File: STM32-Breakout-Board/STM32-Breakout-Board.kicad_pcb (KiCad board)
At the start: 2 copper layers, 32 parts, among them J1 USB_B_Micro, J2 Conn_01x04_Pin, J3 Conn_01x10_Socket, J4 Conn_01x10_Socket, SW1 SW_SPDT, U1 stm32l443cct6, U2 MCP1799T-3302H/DB, Y1 Crystal_GND24

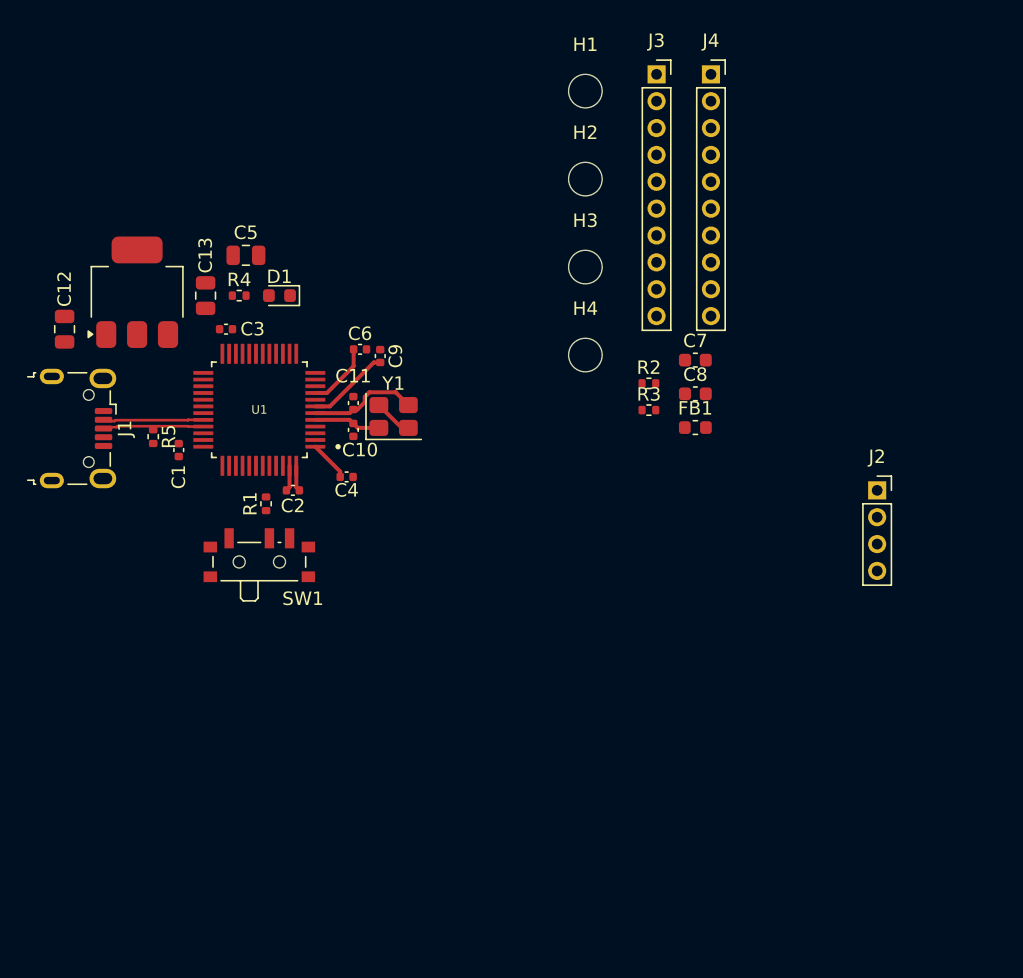
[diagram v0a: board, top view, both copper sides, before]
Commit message: Final Update
Completed layout and Silkscreen decoration
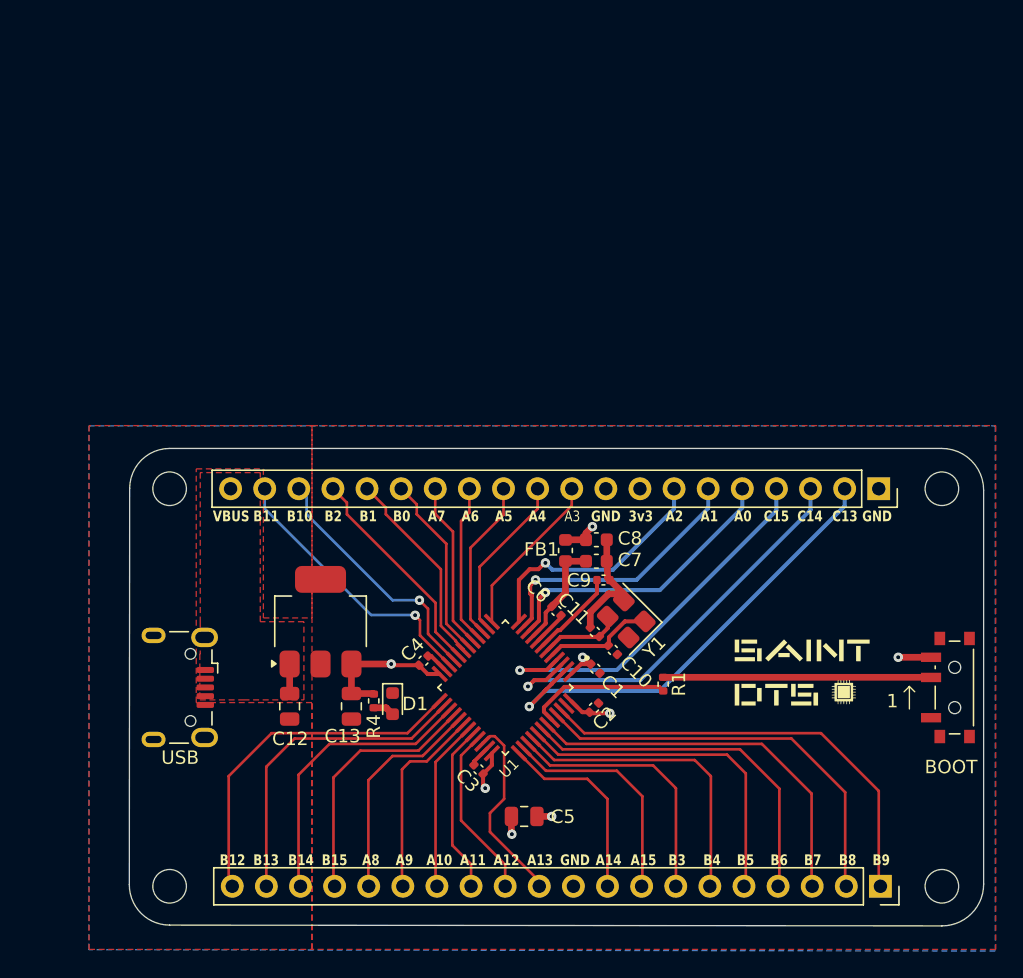
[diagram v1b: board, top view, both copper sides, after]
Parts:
- removed J1: USB_B_Micro, Connector_USB:USB_Micro-B_Wuerth_629105150521
- removed J4: Conn_01x10_Socket, Connector_PinSocket_2.00mm:PinSocket_1x10_P2.00mm_Vertical
- removed R2, R3, R5: 1k5, Resistor_SMD:R_0402_1005Metric
- removed SW1: SW_SPDT, Button_Switch_SMD:SW_SPDT_PCM12
- added BOOT: SW_SPDT, Button_Switch_SMD:SW_SPDT_PCM12, F.Cu at (180.9, 90.7)
- added G***: LOGO, LOGO, F.Cu at (169.9, 89.5)
- added USB: USB_B_Micro, Connector_USB:USB_Micro-B_Wuerth_629105150521, F.Cu at (123.6, 90.7)
- J2: value Conn_01x04_Pin -> Conn_01x20_Pin; footprint Connector_PinSocket_2.00mm:PinSocket_1x04_P2.00mm_Vertical -> Connector_PinHeader_2.54mm:PinHeader_1x20_P2.54mm_Vertical; moved to B.Cu
- J3: value Conn_01x10_Socket -> Conn_01x20_Pin; footprint Connector_PinSocket_2.00mm:PinSocket_1x10_P2.00mm_Vertical -> Connector_PinHeader_2.54mm:PinHeader_1x20_P2.54mm_Vertical; moved to B.Cu
- moved J3 62.7 mm to (175.7, 105.5), turned to 90 degrees
- moved H2 59.0 mm to (180.3, 105.5), turned to -90 degrees
- moved H3 55.5 mm to (122.8, 105.5), turned to -90 degrees
- moved C5 46.6 mm to (149.2, 100.3), turned to 180 degrees
- moved H1 39.8 mm to (180.3, 75.9), turned to -90 degrees
- moved C3 37.8 mm to (145.8, 96.8), turned to 135 degrees
- moved C1 35.0 mm to (154.5, 89.3), turned to -45 degrees
- moved C12 32.7 mm to (131.8, 92.1), turned to -90 degrees
- moved H4 32.5 mm to (122.8, 75.9), turned to -90 degrees
- moved R1 32.5 mm to (159.6, 90.4), turned to -90 degrees
- moved C13 32.4 mm to (136.4, 92.1), turned to -90 degrees
- moved R4 31.8 mm to (138.0, 91.7), turned to -90 degrees
- moved D1 31.5 mm to (139.4, 91.9), turned to -90 degrees
- moved U2 28.1 mm to (134.7, 85.9)
- moved C2 27.6 mm to (154.4, 92.2), turned to 45 degrees
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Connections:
- J2 pad 1: +3.3V -> GND
- J2 pad 2: /I2C_SCL -> /PC13
- J2 pad 3: /I2C_SDA -> /PC14
- J2 pad 4: GND -> /PC15
- J3 pad 1: /PA0 -> /PB9
- J3 pad 10: /PA9 -> GND
- J3 pad 2: /PA1 -> /PB8
- J3 pad 3: /PA2 -> /PB7
- J3 pad 4: /PA3 -> /PB6
- J3 pad 5: /PA4 -> /PB5
- J3 pad 6: /PA5 -> /PB4
- J3 pad 7: /PA6 -> /PB3
- J3 pad 8: /PA7 -> /PA15
- J3 pad 9: /PA8 -> /PA14
- U1 pad 2: unconnected-(U1-PC13-Pad2) -> /PC13
- U1 pad 21: /I2C_SCL -> /PB10
- U1 pad 22: /I2C_SDA -> /PB11
- U1 pad 25: unconnected-(U1-PB12-Pad25) -> /PB12
- U1 pad 26: unconnected-(U1-PB13-Pad26) -> /PB13
- U1 pad 27: unconnected-(U1-PB14-Pad27) -> /PB14
- U1 pad 28: unconnected-(U1-PB15-Pad28) -> /PB15
- U1 pad 3: unconnected-(U1-PC14-Pad3) -> /PC14
- U1 pad 31: unconnected-(U1-PA10-Pad31) -> /PA10
- U1 pad 32: /USB_D- -> /PA11
- U1 pad 33: /USB_D+ -> /PA12
- U1 pad 34: unconnected-(U1-PA13-Pad34) -> /PA13
- U1 pad 37: unconnected-(U1-PA14-Pad37) -> /PA14
- U1 pad 38: unconnected-(U1-PA15-Pad38) -> /PA15
- U1 pad 4: unconnected-(U1-PC15-Pad4) -> /PC15
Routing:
- net /PC13: track 0.00 -> 34.9 mm, vias 0 -> 1
- net /PB9: track 0.00 -> 33.2 mm
- net /PC14: track 0.00 -> 31.2 mm, vias 0 -> 1
- net /PB8: track 0.00 -> 30.9 mm
- net /PC15: track 0.00 -> 28.7 mm, vias 0 -> 1
- net /PB7: track 0.00 -> 28.7 mm
- net /PB6: track 0.00 -> 26.8 mm
- net /PB12: track 0.00 -> 26.3 mm
- net /PB5: track 0.00 -> 25.1 mm
- net /PB13: track 0.00 -> 24.0 mm
- net /PB4: track 0.00 -> 22.6 mm
- net /PA0: track 0.00 -> 22.1 mm, vias 0 -> 1
- net /PB14: track 0.00 -> 21.6 mm
- net +3.3V: track 4.94 -> 26.1 mm, vias 0 -> 7
- net /PB11: track 0.00 -> 20.7 mm, vias 0 -> 1
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- added copper zone on In2.Cu, net +3.3V
- added copper zone on B.Cu, net GND
- added copper zone on F.Cu, net GND
- added copper zone on In1.Cu, net GND
- added copper zone on F.Cu, net VBUS
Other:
- board outline added: 63.6 x 35.6 mm
- copper layers 2 -> 4
- board text added: "1"
- board text added: "3v3"
- board text added: "A0"
- board text added: "A1"
- board text added: "A10"
- board text added: "A11"
- board text added: "A12"
- board text added: "A13"
- board text added: "A14"
- board text added: "A15"
- board text added: "A2"
- board text added: "A3"
- board text added: "A4"
- board text added: "A5"
- board text added: "A6"
- board text added: "A7"
- board text added: "A8"
- board text added: "A9"
- board text added: "B0"
- board text added: "B1"
- board text added: "B10"
- board text added: "B11"
- board text added: "B12"
- board text added: "B13"
- board text added: "B14"
- board text added: "B15"
- board text added: "B2"
- board text added: "B3"
- board text added: "B4"
- board text added: "B5"
- board text added: "B6"
- board text added: "B7"
- board text added: "B8"
- board text added: "B9"
- board text added: "C13"
- board text added: "C14"
- board text added: "C15"
- board text added: "GND"
- board text added: "STM32 Breakout Board By Kidus Ephrem Melaku Revision 0.1"
- board text added: "VBUS"
